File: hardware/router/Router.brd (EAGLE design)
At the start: 133.3 x 101.6 mm, 53 parts, among them J0 CON-MATENLOK, J1 AVR_PROG, J10 RJ45-8PTH, J11 RJ45-8PTH, J12 RJ45-8PTH, J13 RJ45-8PTH, J14 RJ45-8PTH, J15 RJ45-8PTH, J16 RJ45-8PTH, J17 RASPBERRYPI_BB, J18 RJ45-8PTH, J19 RJ45-8PTH, J2 RJ45-8PTH, J3 RJ45-8PTH, J4 RJ45-8PTH, J5 RJ45-8PTH, J6 RJ45-8PTH, J7 RJ45-8PTH, J8 RJ45-8PTH, J9 RJ45-8PTH, Q1 NMOS, Q2 NMOS, Q3 NMOS, U1 ATMEGA168, U3 DS1307SO8, Y1 32.768kHz

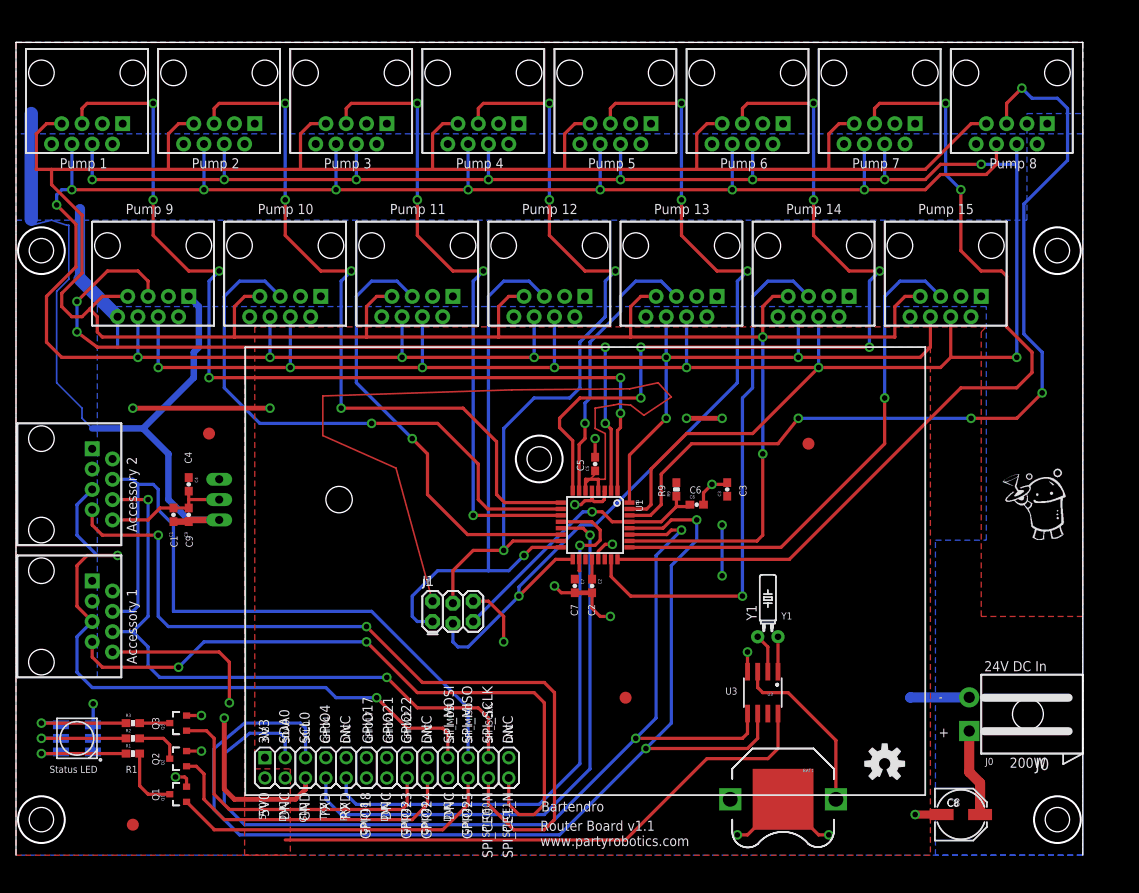
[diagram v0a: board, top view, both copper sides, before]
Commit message: Checking in the latest schematics for the kickstarter
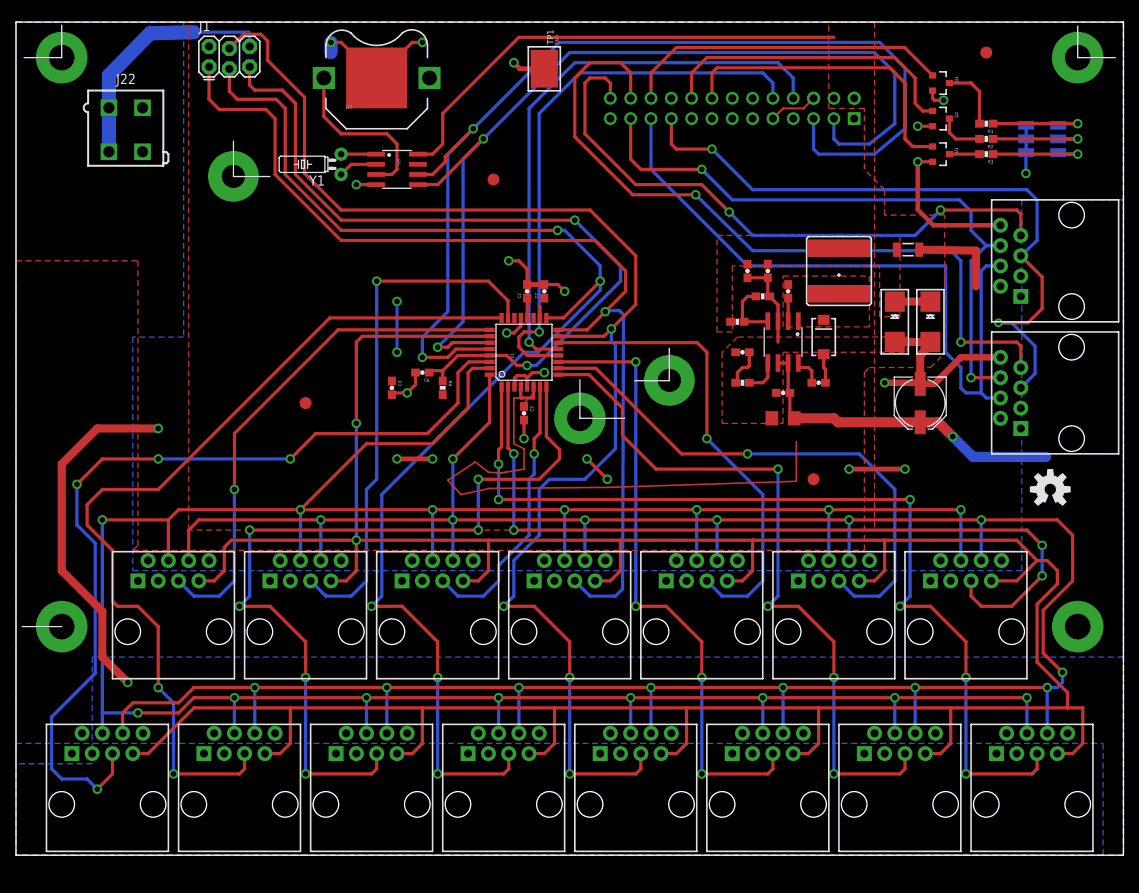
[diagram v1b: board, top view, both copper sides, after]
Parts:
- removed BAT1: 3V, SparkFun-Electromechanical:BATTCON_12MM_PTH
- removed C1: 10u, SparkFun-Passives:0603-CAP
- removed C4: 2.2u, SparkFun-Passives:0603-CAP
- removed C8: 47u, SparkFun-Capacitors:PANASONIC_D
- removed C9: 100n, SparkFun:0603-CAP
- removed J0: CON-MATENLOK, pierre:MINIMATENLOK-2RA
- removed JP5, JP6, JP7, JP8, JP9: STAND-OFFTIGHT, SparkFun-Electromechanical:STAND-OFF-TIGHT
- removed U2: (no value), SparkFun-PowerIC:78XXL
- added C10: 47u, SparkFun-Capacitors:PANASONIC_D
- added C11, C12, C16: 100n, SparkFun:0603-CAP
- added C13: 1u, SparkFun:0603-CAP
- added C14, C17: 1n, SparkFun:0603-CAP
- added C15: 10u, SparkFun-Capacitors:1206
- added C18, C19: 22u, microbuilder:EIA6032-28/C-R
- added D1: 30V3A, pierre:SMA-DIODE
- added F1: PTCSMD, SparkFun-PowerIC:PTC-1206
- added J20: 3V, SparkFun-Electromechanical:BATTCON_12MM_PTH
- added J22: 5566-4, pierre:5566-4
- added L1: 6.8u, pierre:IND_8X8X4
- added R4: 52.3k, SparkFun-Resistors:0603-RES
- added R5, R6: 10k, SparkFun-Resistors:0603-RES
- added TP1: GND, microbuilder:TESTPOINT_SMT
- added U4: AOZ1242SMD, pierre:SO08
- J10, J11, J12, J13, J14, J15, J16, J18, J19, J2, J3, J4, J5, J6, J7, J8, J9: device SparkFun:RJ45-8 -> pierre:RJ45-8
- J17: value RASPBERRYPI_BB -> RASPBERRY-PI_REV2; device pierre:RASBERRYPI_SHIELD -> pierre:RASPBERRY-PI_REV2
- R1, R3: value 300 -> 330
- R2: value 300 -> 200
- moved FRAME3 181.2 mm to (86.6, 158.0), turned to 180 degrees
- moved J2 149.4 mm to (127.0, 6.35), turned to 0 degrees
- moved J9 145.4 mm to (11.4, 6.35), turned to 0 degrees
- moved JP2 143.9 mm to (121.3, 100.3), turned to 180 degrees
- moved LED1 142.0 mm to (128.3, 89.5), turned to 180 degrees
- moved J19 136.2 mm to (132.0, 74.3), turned to 90 degrees
- moved R1 132.6 mm to (121.3, 91.4), turned to 180 degrees
- moved R2 130.4 mm to (121.3, 89.5), turned to 180 degrees
- moved Q1 130.3 mm to (115.6, 96.5), turned to 270 degrees
- moved J18 129.3 mm to (132.0, 57.8), turned to 90 degrees
- moved R3 128.2 mm to (121.3, 87.6), turned to 180 degrees
- moved J3 124.9 mm to (110.5, 6.35), turned to 0 degrees
- moved Q2 124.4 mm to (115.6, 92.1), turned to 270 degrees
- moved J8 121.5 mm to (27.9, 6.35), turned to 0 degrees
- moved Q3 118.9 mm to (115.6, 87.6), turned to 270 degrees
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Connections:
- net RX0 renamed RX8
- net RX7/MOSI renamed RX4/MOSI
- net RX8/MISO renamed RX12/MISO
- net RX9/SCK renamed RX5/SCK
- removed net RX12: J15.5, U1.23
- removed net RX4: J11.5, U1.10
- removed net RX5: J4.5, U1.11
- new net N$15: C14.1, R6.1
- new net N$16: C12.2, D1.C, L1.P$1, U4.1
- new net N$2: R4.1, R5.2, U4.4
- new net N$3: R6.2, U4.5
- new net N$5: C16.1, C17.1, C18.+, C19.+, F1.1, L1.P$2, R4.2
- new net N$7: C12.1, U4.2
- new net N$8: C13.1, U4.8
- new net RX15: J16.5, U1.25
- new net RX7: J8.5, U1.24
- new net RX9: J10.5, U1.2
- net 3.3V: now also J17.P1_1, J17.P1_17; no longer J17.1
- net 5V: now also F1.2, J17.P1_2, J17.P1_4; no longer C4.1, J17.2, U2.OUT
- net BAT1+: now also J20.VCC@1; no longer BAT1.VCC@1
- net BLUE: now also J17.P1_16; no longer J17.16
- net CE0: now also J17.P1_24; no longer J17.24
- net CE1: now also J17.P1_26; no longer J17.26
- net GND: now also C10.-, C11.2, C13.2, C14.2, C15.2, C16.2, C17.2, C18.-, C19.-, D1.A, J17.P1_14, J17.P1_20, J17.P1_25, J17.P1_6, J17.P1_9, J20.GND, J22.1, J22.3, R5.1, TP1.P$1, U4.3; no longer BAT1.GND, C1.2, C4.2, C8.-, C9.2, J0.2, J17.6, U2.GND
- net GREEN: now also J17.P1_22; no longer J17.22
- net RED: now also J17.P1_18; no longer J17.18
- net RPI_MISO: now also J17.P1_21; no longer J17.21
- net RPI_MOSI: now also J17.P1_19; no longer J17.19
- net RPI_RX: now also J17.P1_10; no longer J17.10
- net RPI_SCL: now also J17.P1_5; no longer J17.5
- net RPI_SCLK: now also J17.P1_23; no longer J17.23
- net RPI_SDA: now also J17.P1_3; no longer J17.3
- net RPI_TX: now also J17.P1_8; no longer J17.8
- net RX10: now also J11.5, U1.10; no longer J14.5, U1.7
- net RX11: now also J12.5, U1.14; no longer J7.5, U1.8
- net RX13: now also J14.5, U1.7; no longer J8.5, U1.24
- net RX14: now also J15.5, U1.23; no longer J16.5, U1.25
- net RX2: now also J3.5, U1.9; no longer J10.5, U1.2
- net RX3: now also J4.5, U1.11; no longer J3.5, U1.9
- net RX6: now also J7.5, U1.8; no longer J12.5, U1.14
- net VIN: now also C10.+, C11.1, C15.1, J22.2, J22.4, U4.6, U4.7; no longer C1.1, C8.+, C9.1, J0.1, U2.IN
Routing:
- net RX7: track 0.00 -> 112.2 mm, vias 0 -> 2
- net RX9: track 0.00 -> 101.8 mm, vias 0 -> 4
- net RX5: track 79.7 -> 0.00 mm, vias 4 -> 0
- net RX13: track 112.2 -> 35.0 mm, vias 2 -> 1
- net RX4: track 70.9 -> 0.00 mm, vias 1 -> 0
- net RX4/MOSI: track 100.1 -> 168.4 mm
- net RX12: track 66.1 -> 0.00 mm, vias 1 -> 0
- net VIN: track 107.4 -> 42.4 mm, vias 0 -> 1
- net RX15: track 0.00 -> 64.2 mm, vias 0 -> 1
- net !RST: track 35.6 -> 96.2 mm, vias 1 -> 2
- net RX12/MISO: track 69.3 -> 126.0 mm
- net RX5/SCK: track 113.2 -> 164.7 mm, vias 4 -> 5
- net RX6: track 55.7 -> 103.6 mm, vias 1 -> 6
- net RX11: track 103.6 -> 59.1 mm, vias 6 -> 1
- net GND: track 167.4 -> 210.5 mm, vias 20 -> 22
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- added copper zone on layer 1, net GND
- added copper zone on layer 1, net N$16
- added copper zone on layer 1, net N$5
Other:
- board size 133.3 x 101.6 mm -> 138.4 x 104.1 mm
- board text added: "(c) 2013"
- board text added: "1"
- board text added: "10"
- board text added: "11"
- board text added: "12"
- board text added: "13"
- board text added: "14"
- board text added: "15"
- board text added: "2"
- board text added: "24V DC"
- board text added: "3"
- board text added: "4"
- board text added: "5"
- board text added: "6"
- board text added: "7"
- board text added: "8"
- board text added: "8.3A"
- board text added: "9"
- board text added: "GPIO27"
- board text added: "Router v2"
- board text removed: "200W"
- board text removed: "24V DC In"
- board text removed: "C1"
- board text removed: "C4"
- board text removed: "C8"
- board text removed: "C9"
- board text removed: "DNC"
- board text removed: "GPIO21"
- board text removed: "J0"
- board text removed: "Pump 1"
- board text removed: "Pump 10"
- board text removed: "Pump 11"
- board text removed: "Pump 12"
- board text removed: "Pump 13"
- board text removed: "Pump 14"
- board text removed: "Pump 15"
- board text removed: "Pump 2"
- board text removed: "Pump 3"
- board text removed: "Pump 4"
- board text removed: "Pump 5"
- board text removed: "Pump 6"
- board text removed: "Pump 7"
- board text removed: "Pump 8"
- board text removed: "Pump 9"
- board text removed: "Router Board v1.1"
- board text removed: "Status LED"
- board text removed: "U2"
